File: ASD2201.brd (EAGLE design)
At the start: 22.5 x 22.5 mm, 10 parts, among them J1 DF12-32-DP, J2 DF12-32-DS, J3 DM3D-SF, U1 XC6210B33, U2 TXB0104

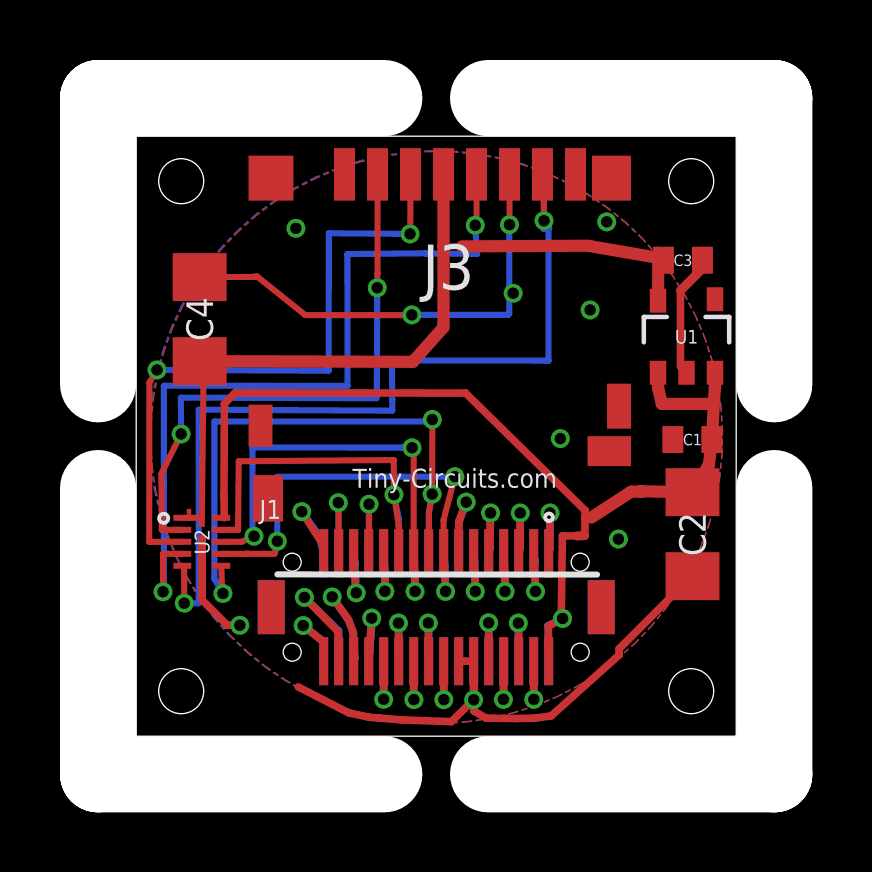
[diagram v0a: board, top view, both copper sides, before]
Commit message: Update for Rev 2 Design
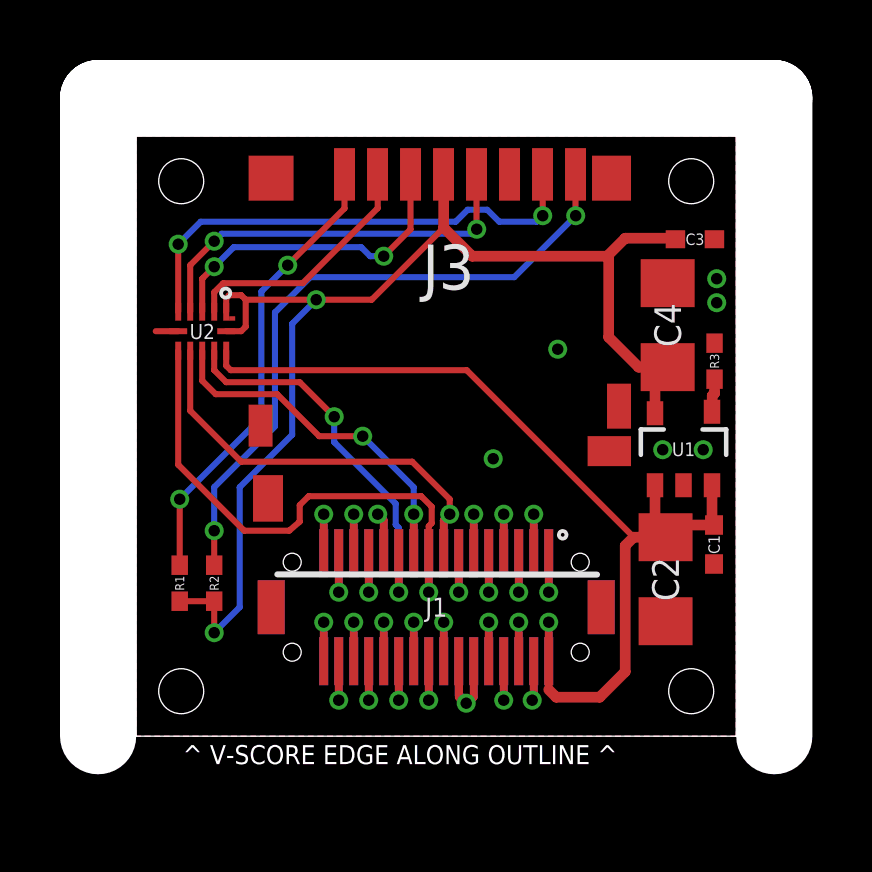
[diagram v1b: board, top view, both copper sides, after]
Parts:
- added R1, R2: 10.0K, tinycircuits:0402
- added R3: 0.0, tinycircuits:0402
- U1: value XC6210B33 -> XC6217A33
- moved C4 15.6 mm to (27.7, 23.7)
- moved U2 7.02 mm to (12.2, 23.5), turned to 180 degrees
- moved U1 3.75 mm to (28.2, 19.6)
- moved C1 3.57 mm to (29.3, 16.4), turned to 270 degrees
- moved C2 1.75 mm to (27.6, 15.2)
- moved C3 0.81 mm to (28.6, 26.6)
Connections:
- new net N$1: J3.1, R1.1
- new net N$2: J3.8, R2.1
- new net N$9: R3.2, U1.4
- net GND: now also R3.1
- net VDD_SD: now also R1.2, R2.2
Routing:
- net GND: track 46.2 -> 9.90 mm, vias 9 -> 7
- net N$2: track 0.00 -> 22.0 mm, vias 0 -> 2
- net N$1: track 0.00 -> 15.3 mm, vias 0 -> 2
- net N$6: track 30.0 -> 16.5 mm
- net VDD_SD: track 29.0 -> 42.1 mm, vias 0 -> 2
- net N$5: track 26.4 -> 13.4 mm
- net N$4: track 22.1 -> 10.8 mm
- net N$3: track 19.3 -> 8.39 mm, vias 2 -> 0
- net VCC: track 37.6 -> 33.7 mm
- net MOSI: track 15.7 -> 13.0 mm, vias 3 -> 2
- net IO3: track 5.22 -> 2.60 mm
- net MISO: track 20.6 -> 18.3 mm, vias 3 -> 1
- net IO2: track 4.70 -> 2.60 mm
- net IO1: track 4.07 -> 2.60 mm
- net N$9: track 0.00 -> 1.12 mm
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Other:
- board size 22.5 x 22.5 mm -> 22.5 x 21.3 mm
- board text added: "2"
- board text added: "ASD2201 - Rev2"
- board text added: "^ V-SCORE EDGE ALONG OUTLINE ^"
- board text added: "microSD TinyShield"
- board text removed: "1"
- board text removed: "ASD2201 - Rev1"
- board text removed: "TinyShield"
- board text removed: "microSD Card"
